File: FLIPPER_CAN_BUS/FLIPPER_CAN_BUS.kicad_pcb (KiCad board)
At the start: 2 copper layers, 62.8 x 21.2 mm, 25 parts, among them J1 Conn_01x02, J2 Conn_01x10_Socket, J3 Conn_01x08_Socket, U1 TJA1051T/3, U2 MCP2515-xST, U3 AP3602AKTR-G1, Y1 16 Mhz

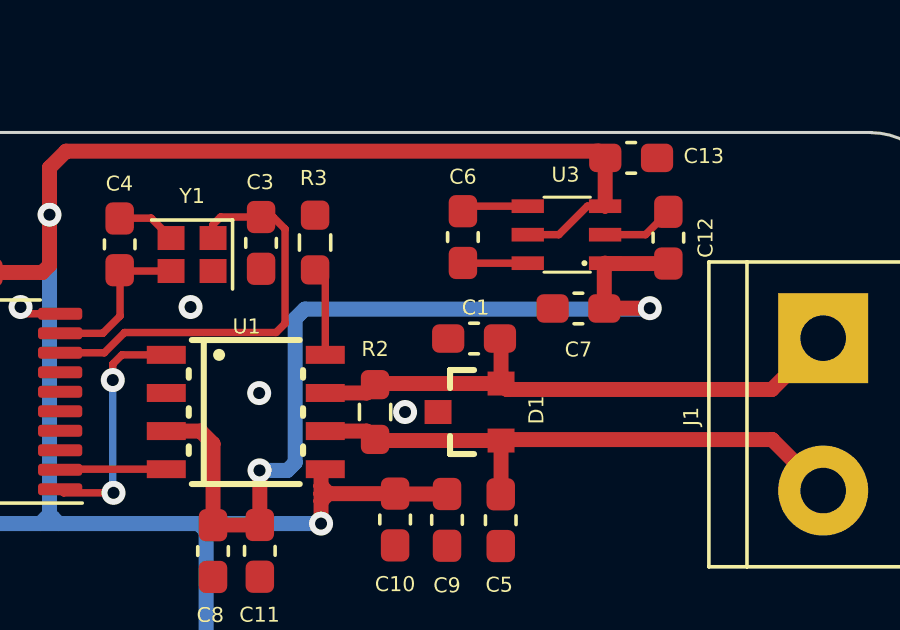
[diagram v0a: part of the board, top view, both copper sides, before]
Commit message: upd PCB
Correcion estetica
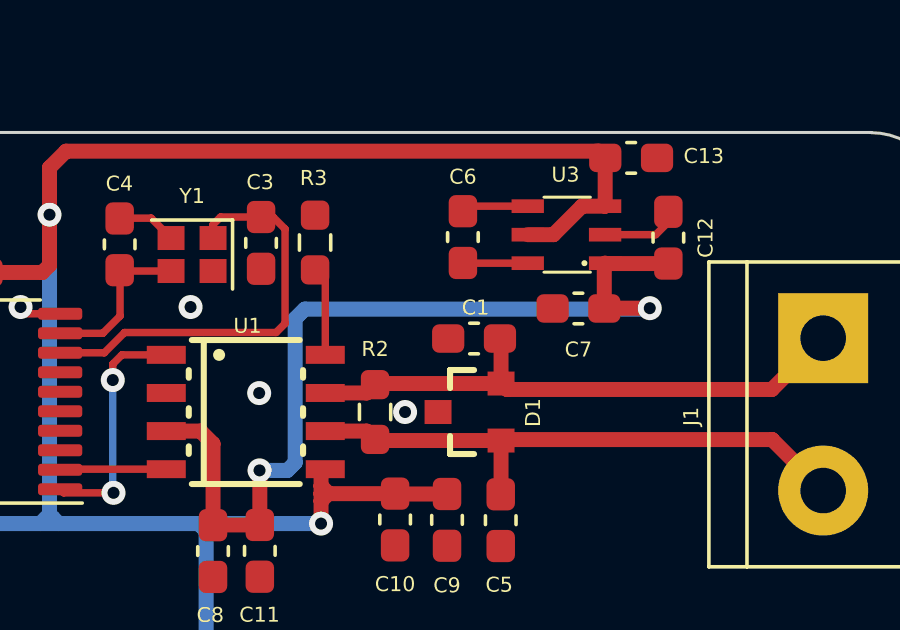
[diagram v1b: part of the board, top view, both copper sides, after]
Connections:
- net /CAN_H+ renamed /CAN_H
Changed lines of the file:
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@@
   (net 31 "unconnected-(J2-Pin_9-Pad9)")
   (net 32 "unconnected-(J3-Pin_1-Pad1)")
-  (net 33 "/CAN_H+")
-  (net 34 "unconnected-(J3-Pin_6-Pad6)")
+  (net 33 "unconnected-(J3-Pin_6-Pad6)")
+  (net 34 "/CAN_H")
   (footprint "Capacitor_SMD:C_0603_1608Metric_Pad1.08x0.95mm_HandSolder" (layer "F.Cu")
     (at 123.421726 85.539223 -90)
@@
       (stroke (width 0.1) (type solid)) (layer "F.Fab"))
     (pad "1" thru_hole rect (at 0 0 270) (size 3 3) (drill 1.52) (layers "*.Cu" "*.Mask")
-      (net 33 "/CAN_H+") (pinfunction "Pin_1") (pintype "passive"))
+      (net 34 "/CAN_H") (pinfunction "Pin_1") (pintype "passive"))
     (pad "2" thru_hole circle (at 5.08 0 270) (size 3 3) (drill 1.52) (layers "*.Cu" "*.Mask")
       (net 1 "/CAN_L") (pinfunction "Pin_2") (pintype "passive"))
@@
       (net 1 "/CAN_L") (pintype "passive"))
     (pad "2" smd roundrect (at 0.9125 0 90) (size 0.975 0.95) (layers "F.Cu" "F.Paste" "F.Mask") (roundrect_rratio 0.25)
-      (net 33 "/CAN_H+") (pintype "passive"))
+      (net 34 "/CAN_H") (pintype "passive"))
     (model "${KICAD6_3DMODEL_DIR}/Resistor_SMD.3dshapes/R_0603_1608Metric.wrl"
       (offset (xyz 0 0 0))
@@
     (property "manf#" "TJA1051T/3,118")
     (attr smd)
-    (fp_text reference "U1" (at -2.851723 -0.027024) (layer "F.SilkS")
+    (fp_text reference "U1" (at -2.871723 -0.057024) (layer "F.SilkS")
         (effects (font (size 0.5 0.5) (thickness 0.125)))
     )
@@
       (net 1 "/CAN_L") (pinfunction "CANL") (pintype "bidirectional"))
     (pad "7" smd rect (at -0.635 -2.65 270) (size 0.6 1.3) (layers "F.Cu" "F.Paste" "F.Mask")
-      (net 33 "/CAN_H+") (pinfunction "CANH") (pintype "bidirectional"))
+      (net 34 "/CAN_H") (pinfunction "CANH") (pintype "bidirectional"))
     (pad "8" smd rect (at -1.905 -2.65 270) (size 0.6 1.3) (layers "F.Cu" "F.Paste" "F.Mask")
       (net 10 "Net-(U1-S)") (pinfunction "S") (pintype "power_in"))
@@
       (stroke (width 0.1) (type solid)) (layer "F.Fab"))
     (pad "1" smd roundrect (at -0.8625 0 180) (size 1.075 0.95) (layers "F.Cu" "F.Paste" "F.Mask") (roundrect_rratio 0.25)
-      (net 33 "/CAN_H+") (pintype "passive"))
+      (net 34 "/CAN_H") (pintype "passive"))
     (pad "2" smd roundrect (at 0.8625 0 180) (size 1.075 0.95) (layers "F.Cu" "F.Paste" "F.Mask") (roundrect_rratio 0.25)
       (net 2 "GND") (pintype "passive"))
@@
     (property "manf#" "PESD1CAN-UX")
     (attr smd)
-    (fp_text reference "D1" (at 0.071723 2.177024 90) (layer "F.SilkS")
+    (fp_text reference "D1" (at -0.018277 2.067024 90) (layer "F.SilkS")
         (effects (font (size 0.5 0.5) (thickness 0.125)))
     )
@@
       (net 1 "/CAN_L") (pinfunction "1") (pintype "bidirectional"))
     (pad "2" smd rect (at 0.95 1 90) (size 0.8 0.9) (layers "F.Cu" "F.Paste" "F.Mask")
-      (net 33 "/CAN_H+") (pinfunction "2") (pintype "bidirectional"))
+      (net 34 "/CAN_H") (pinfunction "2") (pintype "bidirectional"))
     (pad "3" smd rect (at 0 -1.1 90) (size 0.8 0.9) (layers "F.Cu" "F.Paste" "F.Mask")
       (net 2 "GND") (pinfunction "3") (pintype "bidirectional"))
@@
       (net 3 "/SCK") (pinfunction "Pin_5") (pintype "passive"))
     (pad "6" thru_hole oval (at 0 -12.7 270) (size 1.7 1.7) (drill 1) (layers "*.Cu" "*.Mask")
-      (net 34 "unconnected-(J3-Pin_6-Pad6)") (pinfunction "Pin_6") (pintype "passive+no_connect"))
+      (net 33 "unconnected-(J3-Pin_6-Pad6)") (pinfunction "Pin_6") (pintype "passive+no_connect"))
     (pad "7" thru_hole oval (at 0 -15.24 270) (size 1.7 1.7) (drill 1) (layers "*.Cu" "*.Mask")
       (net 6 "/RST") (pinfunction "Pin_7") (pintype "passive"))
@@
   (segment (start 127.300476 81.861723) (end 127.262976 81.824223) (width 0.5) (layer "F.Cu") (net 1))
   (segment (start 115.487976 77.636723) (end 115.262976 77.411723) (width 0.25) (layer "F.Cu") (net 2))
-  (segment (start 137.04155 74.237499) (end 136.27905 74.999999) (width 0.25) (layer "F.Cu") (net 2))
+  (segment (start 136.620001 74.999999) (end 134.9306 74.999999) (width 0.25) (layer "F.Cu") (net 2))
   (segment (start 118.762976 74.449223) (end 119.800476 74.449223) (width 0.25) (layer "F.Cu") (net 2))
   (segment (start 116.765476 77.636723) (end 115.487976 77.636723) (width 0.25) (layer "F.Cu") (net 2))
-  (segment (start 136.27905 74.999999) (end 134.9306 74.999999) (width 0.25) (layer "F.Cu") (net 2))
+  (segment (start 137.04155 74.237499) (end 137.04155 74.57845) (width 0.25) (layer "F.Cu") (net 2))
+  (segment (start 137.04155 74.57845) (end 136.620001 74.999999) (width 0.25) (layer "F.Cu") (net 2))
   (segment (start 119.800476 74.449223) (end 120.462976 75.111723) (width 0.25) (layer "F.Cu") (net 2))
   (segment (start 116.740476 77.611723) (end 116.765476 77.636723) (width 0.25) (layer "F.Cu") (net 2))
@@
   (segment (start 96.2 79.62) (end 96.23 79.65) (width 0.25) (layer "B.Cu") (net 3))
   (segment (start 96.23 79.65) (end 96.23 90.61) (width 0.25) (layer "B.Cu") (net 3))
-  (segment (start 134.9306 74.049998) (end 134.339051 74.049998) (width 0.25) (layer "F.Cu") (net 4))
   (segment (start 116.411376 72.767073) (end 116.961726 72.216723) (width 0.5) (layer "F.Cu") (net 4))
   (segment (start 125.721726 83.631723) (end 125.467976 83.631723) (width 0.5) (layer "F.Cu") (net 4))
@@
   (segment (start 125.717976 83.631723) (end 125.462976 83.376723) (width 0.5) (layer "F.Cu") (net 4))
   (segment (start 116.17 76.26) (end 114.3625 76.26) (width 0.5) (layer "F.Cu") (net 4))
+  (segment (start 134.160002 74.049998) (end 134.9306 74.049998) (width 0.5) (layer "F.Cu") (net 4))
   (segment (start 125.721726 83.631723) (end 125.717976 83.631723) (width 0.5) (layer "F.Cu") (net 4))
   (segment (start 125.721726 83.631723) (end 125.707976 83.631723) (width 0.5) (layer "F.Cu") (net 4))
@@
   (segment (start 125.707976 83.631723) (end 125.462976 83.876723) (width 0.5) (layer "F.Cu") (net 4))
   (segment (start 134.93405 72.539999) (end 134.93405 74.046548) (width 0.5) (layer "F.Cu") (net 4))
-  (segment (start 133.38905 74.999999) (end 132.3525 74.999999) (width 0.25) (layer "F.Cu") (net 4))
+  (segment (start 132.3525 74.999999) (end 133.210001 74.999999) (width 0.5) (layer "F.Cu") (net 4))
   (segment (start 125.462976 82.956723) (end 125.602976 82.816723) (width 0.5) (layer "F.Cu") (net 4))
   (segment (start 125.462976 83.876723) (end 125.462976 83.636723) (width 0.5) (layer "F.Cu") (net 4))
   (segment (start 125.467976 83.631723) (end 125.462976 83.636723) (width 0.5) (layer "F.Cu") (net 4))
-  (segment (start 134.339051 74.049998) (end 133.38905 74.999999) (width 0.25) (layer "F.Cu") (net 4))
   (segment (start 116.411376 74.333923) (end 116.411376 72.767073) (width 0.5) (layer "F.Cu") (net 4))
   (segment (start 116.961726 72.216723) (end 134.713276 72.216723) (width 0.5) (layer "F.Cu") (net 4))
@@
   (segment (start 134.713276 72.216723) (end 134.936551 72.439998) (width 0.5) (layer "F.Cu") (net 4))
   (segment (start 125.462976 83.636723) (end 125.462976 83.376723) (width 0.5) (layer "F.Cu") (net 4))
+  (segment (start 133.210001 74.999999) (end 134.160002 74.049998) (width 0.5) (layer "F.Cu") (net 4))
   (segment (start 127.931726 83.631723) (end 125.721726 83.631723) (width 0.5) (layer "F.Cu") (net 4))
   (segment (start 134.93405 74.046548) (end 134.9306 74.049998) (width 0.5) (layer "F.Cu") (net 4))
@@
   (segment (start 132.3525 74.049998) (end 130.359051 74.049998) (width 0.25) (layer "F.Cu") (net 26))
   (segment (start 130.359051 74.049998) (end 130.19155 74.217499) (width 0.25) (layer "F.Cu") (net 26))
-  (segment (start 126.985476 80.276723) (end 127.262976 79.999223) (width 0.5) (layer "F.Cu") (net 33))
-  (segment (start 131.462976 79.961723) (end 127.300476 79.961723) (width 0.5) (layer "F.Cu") (net 33))
-  (segment (start 131.661253 80.16) (end 131.462976 79.961723) (width 0.5) (layer "F.Cu") (net 33))
-  (segment (start 125.602976 80.276723) (end 126.985476 80.276723) (width 0.5) (layer "F.Cu") (net 33))
-  (segment (start 127.300476 79.961723) (end 127.262976 79.999223) (width 0.5) (layer "F.Cu") (net 33))
-  (segment (start 142.2 78.45) (end 140.49 80.16) (width 0.5) (layer "F.Cu") (net 33))
-  (segment (start 131.462976 79.961723) (end 131.462976 78.499223) (width 0.5) (layer "F.Cu") (net 33))
-  (segment (start 140.49 80.16) (end 131.661253 80.16) (width 0.5) (layer "F.Cu") (net 33))
+  (segment (start 126.985476 80.276723) (end 127.262976 79.999223) (width 0.5) (layer "F.Cu") (net 34))
+  (segment (start 131.462976 79.961723) (end 127.300476 79.961723) (width 0.5) (layer "F.Cu") (net 34))
+  (segment (start 131.661253 80.16) (end 131.462976 79.961723) (width 0.5) (layer "F.Cu") (net 34))
+  (segment (start 125.602976 80.276723) (end 126.985476 80.276723) (width 0.5) (layer "F.Cu") (net 34))
+  (segment (start 127.300476 79.961723) (end 127.262976 79.999223) (width 0.5) (layer "F.Cu") (net 34))
+  (segment (start 142.2 78.45) (end 140.49 80.16) (width 0.5) (layer "F.Cu") (net 34))
+  (segment (start 131.462976 79.961723) (end 131.462976 78.499223) (width 0.5) (layer "F.Cu") (net 34))
+  (segment (start 140.49 80.16) (end 131.661253 80.16) (width 0.5) (layer "F.Cu") (net 34))
   (zone (net 2) (net_name "GND") (layers "F&B.Cu") (hatch edge 0.5)
     (connect_pads (clearance 0.5))
